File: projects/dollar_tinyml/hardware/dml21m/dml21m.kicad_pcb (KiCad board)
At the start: 2 copper layers, 42 x 12 mm, 31 parts, among them J2 Conn_ARM_SWD_TagConnect_TC203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, J4 Header 2.54mm, J5 USB_C_Receptacle_PowerOnly_6P, Q1 BC547B, SW1 PTS647SM50SMTR2LFS, U1 LIS2DH12, U2 Li charger 4054, U3 PY32F003F18U6TR, U4 XC6206P332MR

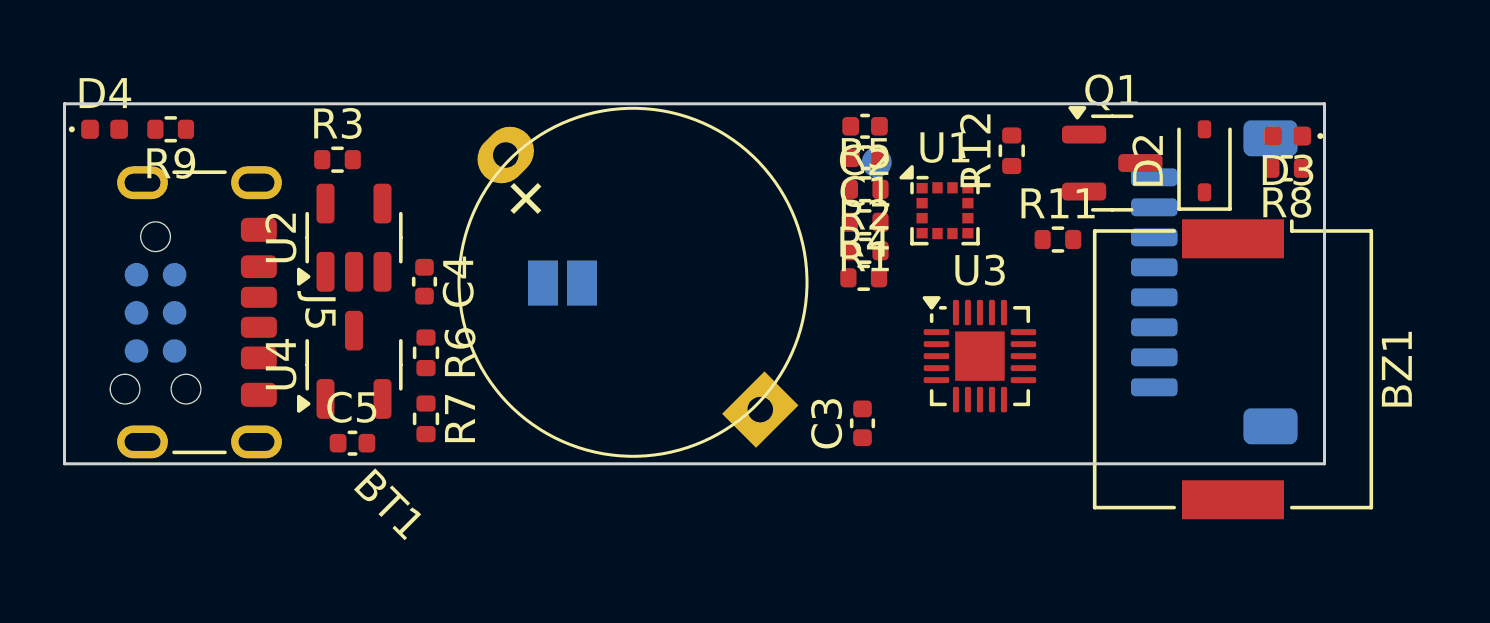
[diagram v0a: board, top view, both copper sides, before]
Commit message: dollarml: More sketches on next board
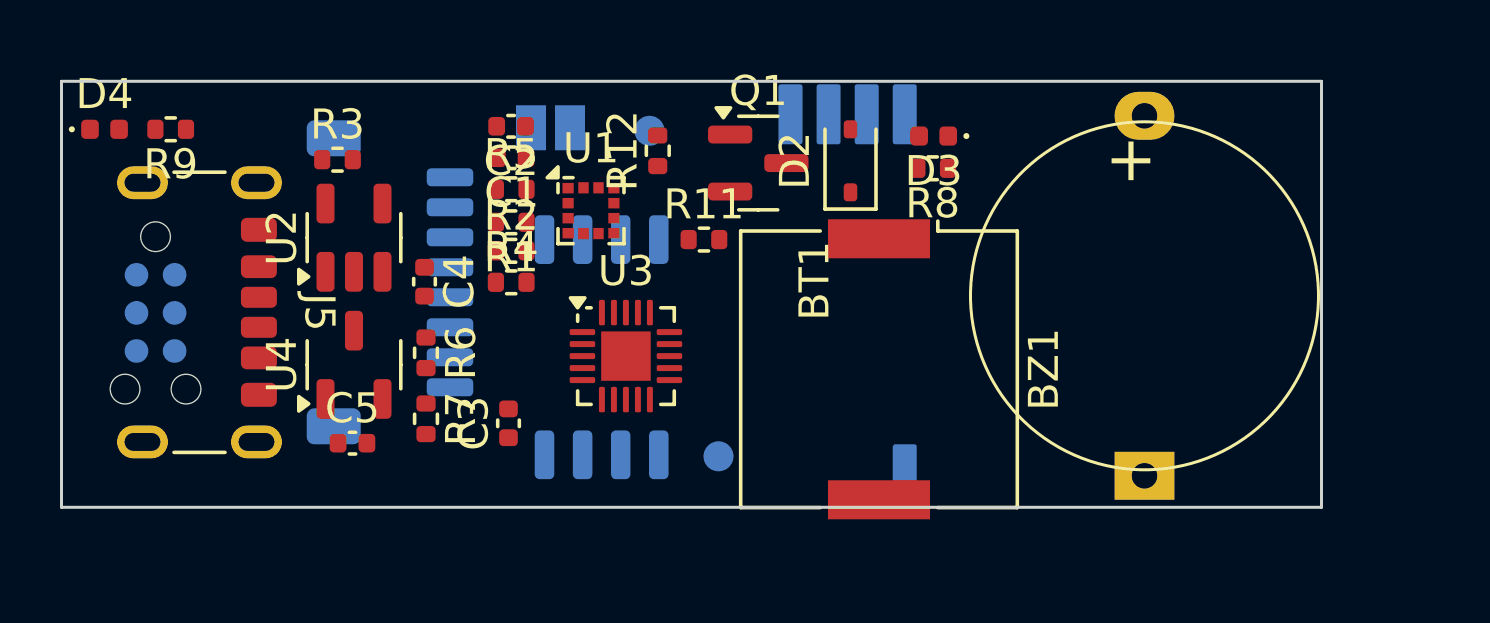
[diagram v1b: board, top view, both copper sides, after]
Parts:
- added TP1: TP_PCB, TestPoint:TestPoint_Pad_D1.0mm, B.Cu at (121.8, 105.8)
- added U5: PUYA P25Q16SH-SSH-IT, Package_SO:SOIC-8_5.3x5.3mm_P1.27mm, B.Cu at (118.0, 102.2)
- added U6: BM7161, dml10:BM7161, B.Cu at (123.2, 100.4)
- BT1: footprint dml21m:Battery_CR1220-Horizontal -> dml20m:Battery_CR1220-Horizontal
- moved J4 27.5 mm to (110.9, 100.0), turned to 90 degrees
- moved BT1 17.1 mm to (136.1, 100.5), turned to 90 degrees
- moved C3 11.8 mm to (114.8, 104.7)
- moved D2 11.8 mm to (126.2, 96.0)
- moved U1 11.8 mm to (117.6, 97.6)
- moved BZ1 11.8 mm to (127.2, 102.9)
- moved C1 11.8 mm to (115.0, 95.8)
- moved C2 11.8 mm to (114.9, 94.8)
- moved Q1 11.8 mm to (123.2, 96.0)
- moved R1 11.8 mm to (114.9, 98.0)
- moved R11 11.8 mm to (121.4, 98.6)
- moved R12 11.8 mm to (119.8, 95.6)
- moved R2 11.8 mm to (114.9, 99.0)
- moved R5 11.8 mm to (114.9, 96.9)
- moved U3 11.8 mm to (118.8, 102.5)
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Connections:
- J4 pad 1: /SWCLK -> /RESET
- J4 pad 2: VDD -> /SWCLK
- J4 pad 3: GND -> VDD
- J4 pad 4: /SDA -> GND
- J4 pad 5: /SCL -> /SDA
- J4 pad 6: /SWDIO -> /SCL
- J4 pad 7: (no net) -> /SWDIO
- J4 pad 8: (no net) -> unconnected-(J4-Pin_8-Pad8)
- U3 pad 3: /LED_RED_P -> unconnected-(U3-PA7-Pad3)
- U3 pad 5: /LED_BLUE_P -> unconnected-(U3-PA12-Pad5)
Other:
- board size 42 x 12 mm -> 42 x 14.2 mm
